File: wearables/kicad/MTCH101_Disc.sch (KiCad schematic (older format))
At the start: 15 parts, among them U1 MTCH101_PKG

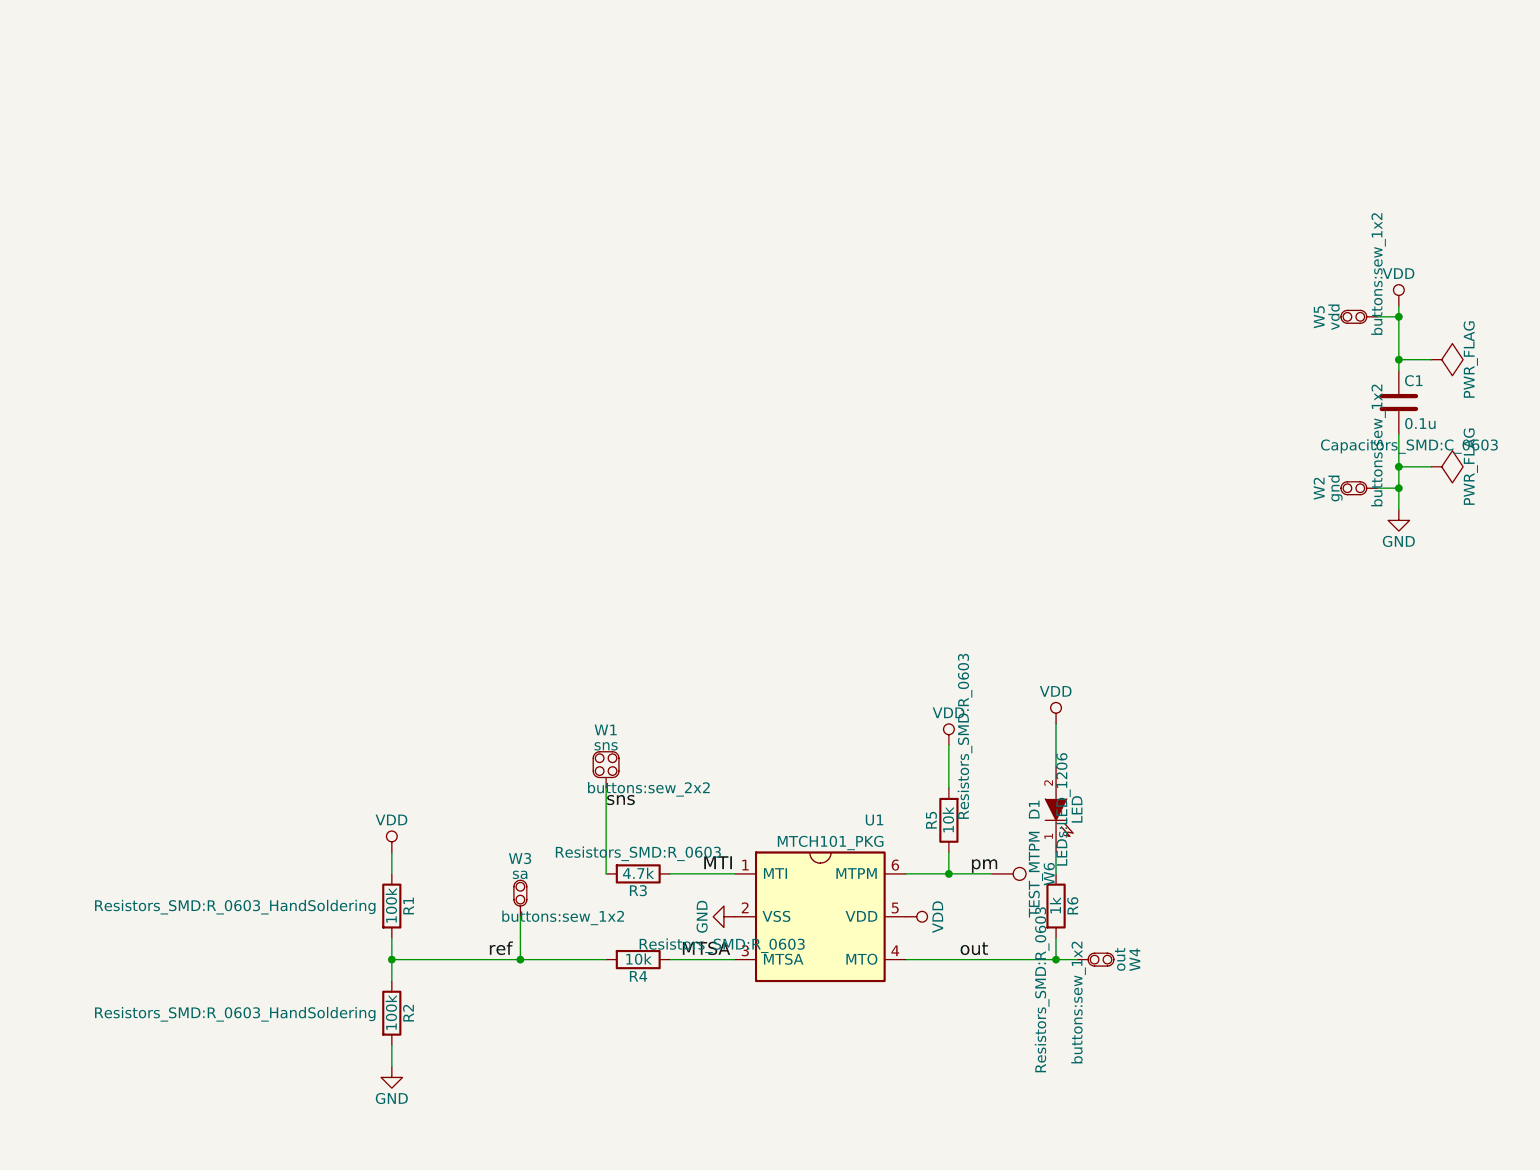
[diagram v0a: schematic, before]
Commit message: more dabbling
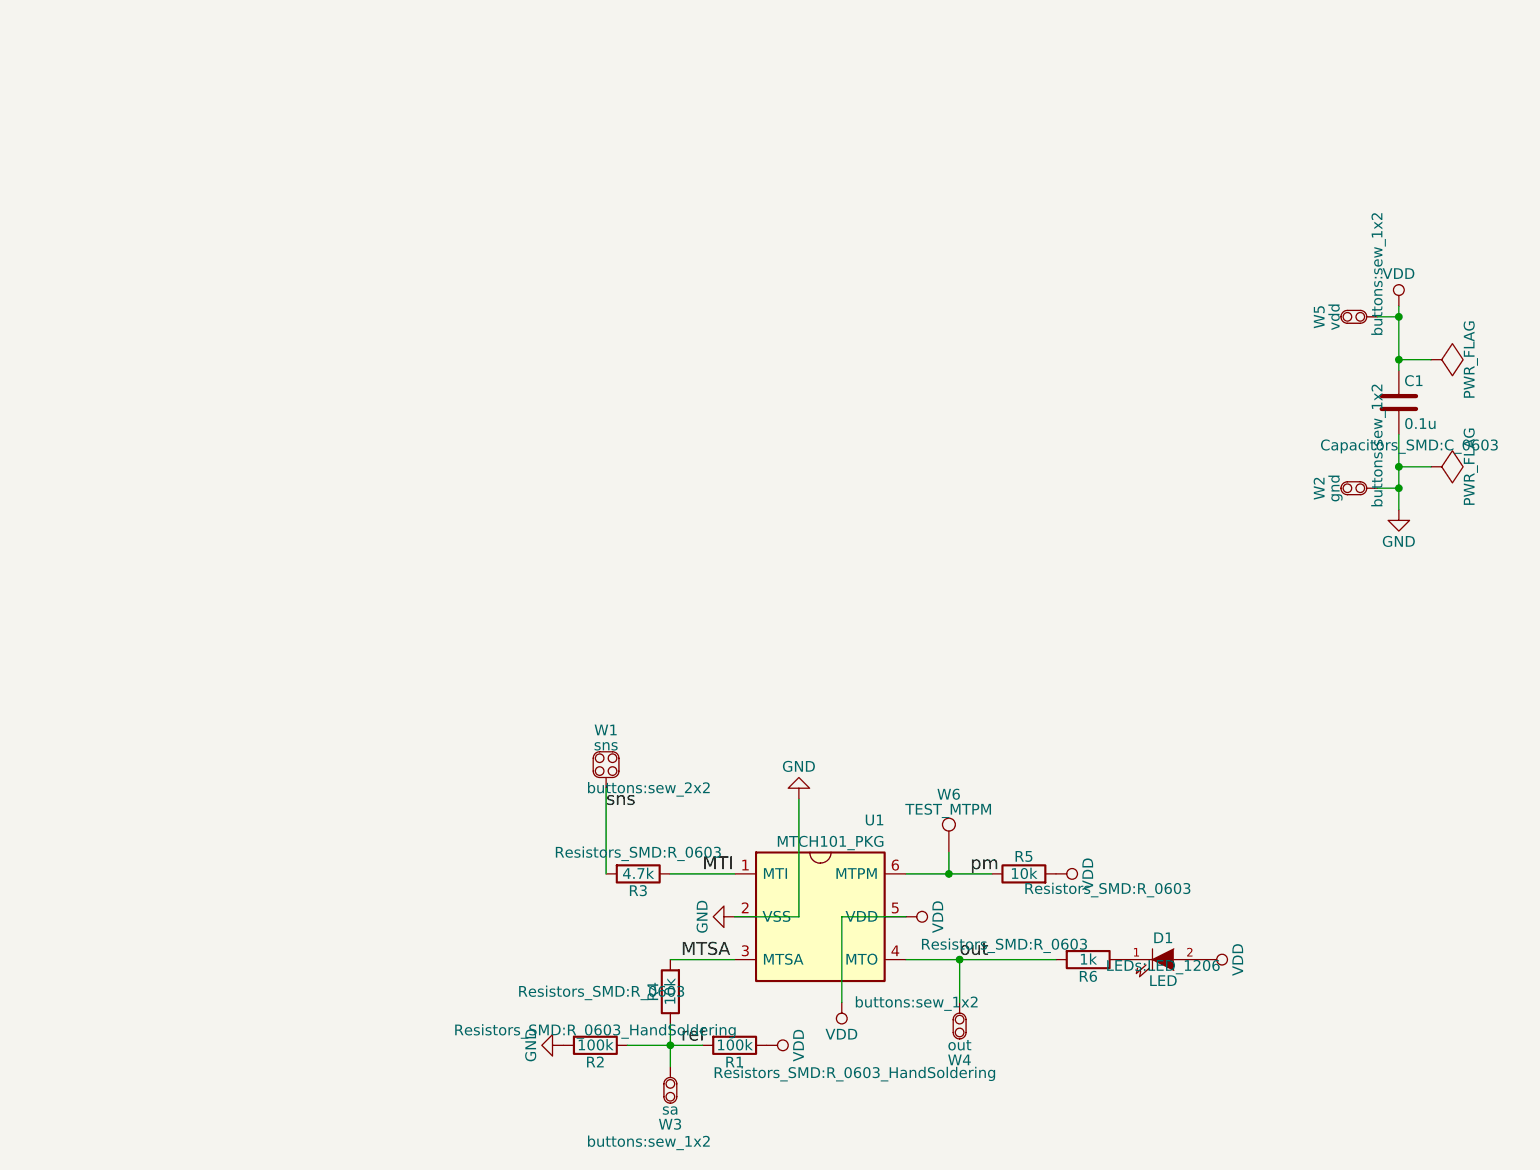
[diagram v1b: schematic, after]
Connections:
- net MTSA: now also R4.2; no longer R4.1
- net ref: now also R4.1; no longer R4.2
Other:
- moved on the sheet: D1, R1, R2, R4, R5, R6, W3, W4, W6
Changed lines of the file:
@@
 L R R4
 U 1 1 58064DD0
-P 3450 5600
-F 0 "R4" V 3530 5600 50  0000 C CNN
-F 1 "10k" V 3450 5600 50  0000 C CNN
-F 2 "Resistors_SMD:R_0603" V 3380 5600 50  0000 L CNN
-F 3 "" H 3450 5600 50  0000 C CNN
-	1    3450 5600
-	0    1    1    0
+P 3600 5750
+F 0 "R4" V 3680 5750 50  0000 C CNN
+F 1 "10k" V 3600 5750 50  0000 C CNN
+F 2 "Resistors_SMD:R_0603" H 3530 5750 50  0000 L CNN
+F 3 "" H 3600 5750 50  0000 C CNN
+	1    3600 5750
+	-1   0    0    1
 $EndComp
 $Comp
 L R R5
 U 1 1 58064FBC
-P 4900 4950
-F 0 "R5" V 4980 4950 50  0000 C CNN
-F 1 "10k" V 4900 4950 50  0000 C CNN
-F 2 "Resistors_SMD:R_0603" V 4830 4950 50  0000 R CNN
-F 3 "" H 4900 4950 50  0000 C CNN
-	1    4900 4950
-	-1   0    0    1
+P 5250 5200
+F 0 "R5" V 5330 5200 50  0000 C CNN
+F 1 "10k" V 5250 5200 50  0000 C CNN
+F 2 "Resistors_SMD:R_0603" V 5180 5200 50  0000 R CNN
+F 3 "" H 5250 5200 50  0000 C CNN
+	1    5250 5200
+	0    -1   -1   0
 $EndComp
 $Comp
 L R R1
 U 1 1 580650CE
-P 2300 5350
-F 0 "R1" V 2380 5350 50  0000 C CNN
-F 1 "100k" V 2300 5350 50  0000 C CNN
-F 2 "Resistors_SMD:R_0603_HandSoldering" H 2230 5350 50  0000 R CNN
-F 3 "" H 2300 5350 50  0000 C CNN
-	1    2300 5350
-	1    0    0    -1
+P 3900 6000
+F 0 "R1" V 3980 6000 50  0000 C CNN
+F 1 "100k" V 3900 6000 50  0000 C CNN
+F 2 "Resistors_SMD:R_0603_HandSoldering" V 4000 5900 50  0000 L TNN
+F 3 "" H 3900 6000 50  0000 C CNN
+	1    3900 6000
+	0    1    1    0
 $EndComp
 $Comp
 L R R2
 U 1 1 580650FF
-P 2300 5850
-F 0 "R2" V 2380 5850 50  0000 C CNN
-F 1 "100k" V 2300 5850 50  0000 C CNN
-F 2 "Resistors_SMD:R_0603_HandSoldering" H 2230 5850 50  0000 R CNN
-F 3 "" H 2300 5850 50  0000 C CNN
-	1    2300 5850
-	1    0    0    -1
+P 3250 6000
+F 0 "R2" V 3330 6000 50  0000 C CNN
+F 1 "100k" V 3250 6000 50  0000 C CNN
+F 2 "Resistors_SMD:R_0603_HandSoldering" V 3180 6000 50  0000 C CNN
+F 3 "" H 3250 6000 50  0000 C CNN
+	1    3250 6000
+	0    1    1    0
 $EndComp
 $Comp
@@
 L R R6
 U 1 1 58065673
-P 5400 5350
-F 0 "R6" V 5480 5350 50  0000 C CNN
-F 1 "1k" V 5400 5350 50  0000 C CNN
-F 2 "Resistors_SMD:R_0603" V 5330 5350 50  0000 R CNN
-F 3 "" H 5400 5350 50  0000 C CNN
-	1    5400 5350
-	1    0    0    -1
+P 5550 5600
+F 0 "R6" V 5630 5600 50  0000 C CNN
+F 1 "1k" V 5550 5600 50  0000 C CNN
+F 2 "Resistors_SMD:R_0603" V 5480 5600 50  0000 R CNN
+F 3 "" H 5550 5600 50  0000 C CNN
+	1    5550 5600
+	0    1    1    0
 $EndComp
 $Comp
 L LED D1
 U 1 1 5806579A
-P 5400 4900
-F 0 "D1" H 5400 5000 50  0000 C CNN
-F 1 "LED" H 5400 4800 50  0000 C CNN
-F 2 "LEDs:LED_1206" H 5400 4900 50  0000 C TNN
-F 3 "" H 5400 4900 50  0000 C CNN
-	1    5400 4900
-	0    -1   -1   0
+P 5900 5600
+F 0 "D1" H 5900 5700 50  0000 C CNN
+F 1 "LED" H 5900 5500 50  0000 C CNN
+F 2 "LEDs:LED_1206" H 5900 5600 50  0000 C TNN
+F 3 "" H 5900 5600 50  0000 C CNN
+	1    5900 5600
+	1    0    0    -1
 $EndComp
 Text Label 4950 5600 0    60   ~ 0
@@
 Text Label 3300 4900 0    60   ~ 0
 sns
-Text Label 2750 5600 0    60   ~ 0
+Text Label 3650 6000 0    60   ~ 0
 ref
 $Comp
 L TEST_1P W6
 U 1 1 580662C8
-P 5100 5200
-F 0 "W6" H 5100 5470 50  0000 C CNN
-F 1 "TEST_MTPM" H 5100 5400 50  0000 C CNN
-F 2 "Measurement_Points:Measurement_Point_Round-SMD-Pad_Small" H 5300 5200 50  0001 C CNN
-F 3 "" H 5300 5200 50  0000 C CNN
-	1    5100 5200
-	0    1    1    0
+P 4900 5100
+F 0 "W6" H 4900 5370 50  0000 C CNN
+F 1 "TEST_MTPM" H 4900 5300 50  0000 C CNN
+F 2 "Measurement_Points:Measurement_Point_Round-SMD-Pad_Small" H 5100 5100 50  0001 C CNN
+F 3 "" H 5100 5100 50  0000 C CNN
+	1    4900 5100
+	1    0    0    -1
 $EndComp
 $Comp
 L VDD #vdd03
 U 1 1 58067C71
-P 5400 4500
-F 0 "#vdd03" H 5400 4350 50  0001 C CNN
-F 1 "VDD" H 5400 4650 50  0000 C CNN
-F 2 "" H 5400 4500 50  0000 C CNN
-F 3 "" H 5400 4500 50  0000 C CNN
-	1    5400 4500
-	1    0    0    -1
+P 6100 5600
+F 0 "#vdd03" H 6100 5450 50  0001 C CNN
+F 1 "VDD" H 6100 5750 50  0000 C CNN
+F 2 "" H 6100 5600 50  0000 C CNN
+F 3 "" H 6100 5600 50  0000 C CNN
+	1    6100 5600
+	0    1    1    0
 $EndComp
 $Comp
 L VDD #vdd04
 U 1 1 580681E5
-P 4900 4600
-F 0 "#vdd04" H 4900 4450 50  0001 C CNN
-F 1 "VDD" H 4900 4750 50  0000 C CNN
-F 2 "" H 4900 4600 50  0000 C CNN
-F 3 "" H 4900 4600 50  0000 C CNN
-	1    4900 4600
-	1    0    0    -1
+P 5400 5200
+F 0 "#vdd04" H 5400 5050 50  0001 C CNN
+F 1 "VDD" H 5400 5350 50  0000 C CNN
+F 2 "" H 5400 5200 50  0000 C CNN
+F 3 "" H 5400 5200 50  0000 C CNN
+	1    5400 5200
+	0    1    1    0
 $EndComp
 $Comp
@@
 L VDD #vdd06
 U 1 1 58068249
-P 2300 5100
-F 0 "#vdd06" H 2300 4950 50  0001 C CNN
-F 1 "VDD" H 2300 5250 50  0000 C CNN
-F 2 "" H 2300 5100 50  0000 C CNN
-F 3 "" H 2300 5100 50  0000 C CNN
-	1    2300 5100
-	1    0    0    -1
+P 4050 6000
+F 0 "#vdd06" H 4050 5850 50  0001 C CNN
+F 1 "VDD" H 4050 6150 50  0000 C CNN
+F 2 "" H 4050 6000 50  0000 C CNN
+F 3 "" H 4050 6000 50  0000 C CNN
+	1    4050 6000
+	0    1    1    0
 $EndComp
 $Comp
@@
 L GND #gnd08
 U 1 1 580686F1
-P 2300 6100
-F 0 "#gnd08" H 2300 5850 50  0001 C CNN
-F 1 "GND" H 2300 5950 50  0000 C CNN
-F 2 "" H 2300 6100 50  0000 C CNN
-F 3 "" H 2300 6100 50  0000 C CNN
-	1    2300 6100
-	1    0    0    -1
+P 3100 6000
+F 0 "#gnd08" H 3100 5750 50  0001 C CNN
+F 1 "GND" H 3100 5850 50  0000 C CNN
+F 2 "" H 3100 6000 50  0000 C CNN
+F 3 "" H 3100 6000 50  0000 C CNN
+	1    3100 6000
+	0    1    1    0
 $EndComp
 $Comp
@@
 	4700 5200 5100 5200
 Wire Wire Line
-	2300 5500 2300 5700
-Wire Wire Line
-	2300 5600 3300 5600
-Connection ~ 2300 5600
-Wire Wire Line
-	2300 5100 2300 5200
-Wire Wire Line
-	2300 6000 2300 6100
-Wire Wire Line
-	5400 5600 5400 5500
-Wire Wire Line
-	5400 5100 5400 5200
-Wire Wire Line
-	5400 4500 5400 4700
-Wire Wire Line
-	4700 5600 5500 5600
-Connection ~ 5400 5600
-Wire Wire Line
-	4900 4600 4900 4800
+	4700 5600 5400 5600
 Wire Wire Line
 	4900 5100 4900 5200
 Connection ~ 4900 5200
-Wire Wire Line
-	2900 5600 2900 5600
-Connection ~ 2900 5600
 Wire Wire Line
 	7150 2800 7000 2800
@@
 Wire Wire Line
 	3600 5600 3900 5600
-Wire Wire Line
-	2900 5400 2900 5600
 $Comp
 L SEW_1X2 W3
 U 1 1 580A30E6
-P 2900 5400
-F 0 "W3" H 2900 5670 50  0000 C CNN
-F 1 "sa" H 2900 5600 50  0000 C CNN
-F 2 "buttons:sew_1x2" H 3100 5400 50  0000 C CNN
-F 3 "" H 3100 5400 50  0000 C CNN
-	1    2900 5400
-	1    0    0    -1
+P 3600 6100
+F 0 "W3" H 3600 6370 50  0000 C CNN
+F 1 "sa" H 3600 6300 50  0000 C CNN
+F 2 "buttons:sew_1x2" H 3700 6450 50  0000 C CNN
+F 3 "" H 3800 6100 50  0000 C CNN
+	1    3600 6100
+	-1   0    0    1
 $EndComp
 $Comp
 L SEW_1X2 W4
 U 1 1 580A3684
-P 5500 5600
-F 0 "W4" H 5500 5870 50  0000 C CNN
-F 1 "out" H 5500 5800 50  0000 C CNN
-F 2 "buttons:sew_1x2" H 5700 5600 50  0000 C CNN
-F 3 "" H 5700 5600 50  0000 C CNN
-	1    5500 5600
-	0    1    1    0
+P 4950 5800
+F 0 "W4" H 4950 6070 50  0000 C CNN
+F 1 "out" H 4950 6000 50  0000 C CNN
+F 2 "buttons:sew_1x2" H 5150 5800 50  0000 C CNN
+F 3 "" H 5150 5800 50  0000 C CNN
+	1    4950 5800
+	-1   0    0    1
 $EndComp
 $Comp
@@
 	0    -1   -1   0
 $EndComp
+Wire Wire Line
+	4950 5800 4950 5600
+Connection ~ 4950 5600
+Wire Wire Line
+	3600 5900 3600 6100
+Wire Wire Line
+	3400 6000 3750 6000
+Connection ~ 3600 6000
+$Comp
+L GND #gnd011
+U 1 1 580A55A8
+P 4200 4850
+F 0 "#gnd011" H 4200 4600 50  0001 C CNN
+F 1 "GND" H 4200 4700 50  0000 C CNN
+F 2 "" H 4200 4850 50  0000 C CNN
+F 3 "" H 4200 4850 50  0000 C CNN
+	1    4200 4850
+	-1   0    0    1
+$EndComp
+Wire Wire Line
+	3900 5400 4200 5400
+Wire Wire Line
+	4200 5400 4200 4850
+$Comp
+L VDD #vdd012
+U 1 1 580A5607
+P 4400 5800
+F 0 "#vdd012" H 4400 5650 50  0001 C CNN
+F 1 "VDD" H 4400 5950 50  0000 C CNN
+F 2 "" H 4400 5800 50  0000 C CNN
+F 3 "" H 4400 5800 50  0000 C CNN
+	1    4400 5800
+	-1   0    0    1
+$EndComp
+Wire Wire Line
+	4700 5400 4400 5400
+Wire Wire Line
+	4400 5400 4400 5800
 $EndSCHEMATC

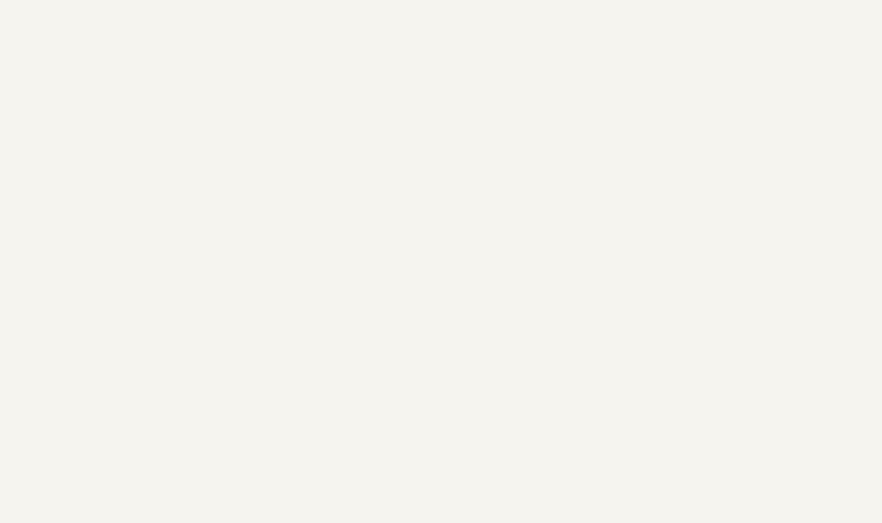
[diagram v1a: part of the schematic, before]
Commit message: More misc play.
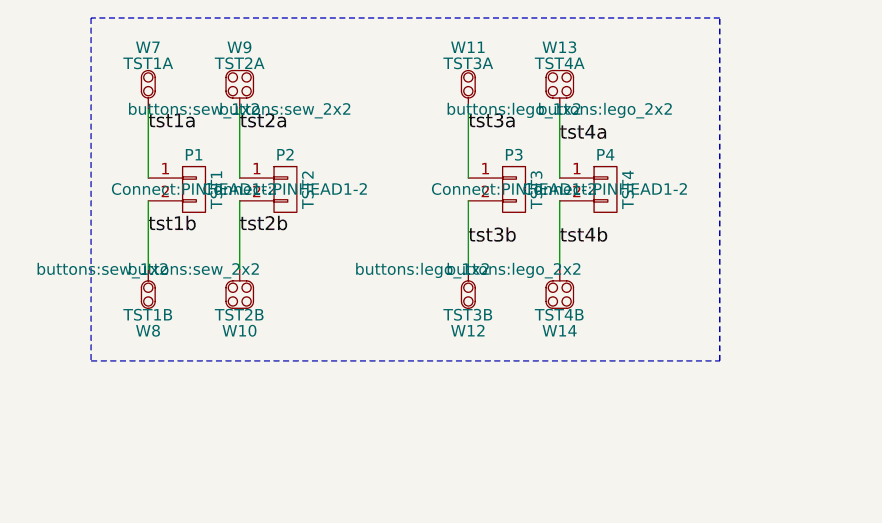
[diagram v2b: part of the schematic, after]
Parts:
- added P1: TST1, Connect:PINHEAD1-2, symbol CONN_01X02
- added P2: TST2, Connect:PINHEAD1-2, symbol CONN_01X02
- added P3: TST3, Connect:PINHEAD1-2, symbol CONN_01X02
- added P4: TST4, Connect:PINHEAD1-2, symbol CONN_01X02
- added W10: TST2B, buttons:sew_2x2, symbol SEW_2X2
- added W11: TST3A, buttons:lego_1x2, symbol SEW_1X2
- added W12: TST3B, buttons:lego_1x2, symbol SEW_1X2
- added W13: TST4A, buttons:lego_2x2, symbol SEW_2X2
- added W14: TST4B, buttons:lego_2x2, symbol SEW_2X2
- added W7: TST1A, buttons:sew_1x2, symbol SEW_1X2
- added W8: TST1B, buttons:sew_1x2, symbol SEW_1X2
- added W9: TST2A, buttons:sew_2x2, symbol SEW_2X2
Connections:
- new net tst1a: P1.1 (P1), W7.1
- new net tst1b: P1.2 (P2), W8.1
- new net tst2a: P2.1 (P1), W9.1
- new net tst2b: P2.2 (P2), W10.1
- new net tst3a: P3.1 (P1), W11.1
- new net tst3b: P3.2 (P2), W12.1
- new net tst4a: P4.1 (P1), W13.1
- new net tst4b: P4.2 (P2), W14.1
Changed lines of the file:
@@
 Wire Wire Line
 	4400 5400 4400 5800
+Wire Notes Line
+	4100 1200 1350 1200
+Wire Notes Line
+	1350 1200 1350 2700
+Wire Notes Line
+	1350 2700 4100 2700
+Wire Notes Line
+	4100 2700 4100 1200
+$Comp
+L SEW_1X2 W7
+U 1 1 580CE257
+P 1600 1600
+F 0 "W7" H 1600 1870 50  0000 C CNN
+F 1 "TST1A" H 1600 1800 50  0000 C CNN
+F 2 "buttons:sew_1x2" H 1800 1600 50  0000 C CNN
+F 3 "" H 1800 1600 50  0000 C CNN
+	1    1600 1600
+	1    0    0    -1
+$EndComp
+$Comp
+L SEW_1X2 W8
+U 1 1 580CE2C7
+P 1600 2300
+F 0 "W8" H 1600 2570 50  0000 C CNN
+F 1 "TST1B" H 1600 2500 50  0000 C CNN
+F 2 "buttons:sew_1x2" H 1800 2300 50  0000 C CNN
+F 3 "" H 1800 2300 50  0000 C CNN
+	1    1600 2300
+	-1   0    0    1
+$EndComp
+$Comp
+L SEW_2X2 W9
+U 1 1 580CE33E
+P 2000 1600
+F 0 "W9" H 2000 1870 50  0000 C CNN
+F 1 "TST2A" H 2000 1800 50  0000 C CNN
+F 2 "buttons:sew_2x2" H 2200 1600 50  0000 C CNN
+F 3 "" H 2200 1600 50  0000 C CNN
+	1    2000 1600
+	1    0    0    -1
+$EndComp
+$Comp
+L SEW_2X2 W10
+U 1 1 580CE39E
+P 2000 2300
+F 0 "W10" H 2000 2570 50  0000 C CNN
+F 1 "TST2B" H 2000 2500 50  0000 C CNN
+F 2 "buttons:sew_2x2" H 2200 2300 50  0000 C CNN
+F 3 "" H 2200 2300 50  0000 C CNN
+	1    2000 2300
+	-1   0    0    1
+$EndComp
+Wire Wire Line
+	1600 1600 1600 1900
+Wire Wire Line
+	2000 1600 2000 1900
+Wire Wire Line
+	2000 2000 2000 2300
+Wire Wire Line
+	1600 2000 1600 2300
+$Comp
+L CONN_01X02 P1
+U 1 1 580CE890
+P 1800 1950
+F 0 "P1" H 1800 2100 50  0000 C CNN
+F 1 "TST1" V 1900 1950 50  0000 C CNN
+F 2 "Connect:PINHEAD1-2" H 1800 1950 50  0000 C CNN
+F 3 "" H 1800 1950 50  0000 C CNN
+	1    1800 1950
+	1    0    0    -1
+$EndComp
+$Comp
+L CONN_01X02 P2
+U 1 1 580CE8EA
+P 2200 1950
+F 0 "P2" H 2200 2100 50  0000 C CNN
+F 1 "TST2" V 2300 1950 50  0000 C CNN
+F 2 "Connect:PINHEAD1-2" H 2200 1950 50  0000 C CNN
+F 3 "" H 2200 1950 50  0000 C CNN
+	1    2200 1950
+	1    0    0    -1
+$EndComp
+$Comp
+L SEW_1X2 W11
+U 1 1 580CF0AD
+P 3000 1600
+F 0 "W11" H 3000 1870 50  0000 C CNN
+F 1 "TST3A" H 3000 1800 50  0000 C CNN
+F 2 "buttons:lego_1x2" H 3200 1600 50  0000 C CNN
+F 3 "" H 3200 1600 50  0000 C CNN
+	1    3000 1600
+	1    0    0    -1
+$EndComp
+$Comp
+L SEW_1X2 W12
+U 1 1 580CF0B3
+P 3000 2300
+F 0 "W12" H 3000 2570 50  0000 C CNN
+F 1 "TST3B" H 3000 2500 50  0000 C CNN
+F 2 "buttons:lego_1x2" H 3200 2300 50  0000 C CNN
+F 3 "" H 3200 2300 50  0000 C CNN
+	1    3000 2300
+	-1   0    0    1
+$EndComp
+$Comp
+L SEW_2X2 W13
+U 1 1 580CF0B9
+P 3400 1600
+F 0 "W13" H 3400 1870 50  0000 C CNN
+F 1 "TST4A" H 3400 1800 50  0000 C CNN
+F 2 "buttons:lego_2x2" H 3600 1600 50  0000 C CNN
+F 3 "" H 3600 1600 50  0000 C CNN
+	1    3400 1600
+	1    0    0    -1
+$EndComp
+$Comp
+L SEW_2X2 W14
+U 1 1 580CF0BF
+P 3400 2300
+F 0 "W14" H 3400 2570 50  0000 C CNN
+F 1 "TST4B" H 3400 2500 50  0000 C CNN
+F 2 "buttons:lego_2x2" H 3600 2300 50  0000 C CNN
+F 3 "" H 3600 2300 50  0000 C CNN
+	1    3400 2300
+	-1   0    0    1
+$EndComp
+Wire Wire Line
+	3000 1600 3000 1900
+Wire Wire Line
+	3400 1600 3400 1900
+Wire Wire Line
+	3400 2000 3400 2300
+Wire Wire Line
+	3000 2000 3000 2300
+$Comp
+L CONN_01X02 P3
+U 1 1 580CF0C9
+P 3200 1950
+F 0 "P3" H 3200 2100 50  0000 C CNN
+F 1 "TST3" V 3300 1950 50  0000 C CNN
+F 2 "Connect:PINHEAD1-2" H 3200 1950 50  0000 C CNN
+F 3 "" H 3200 1950 50  0000 C CNN
+	1    3200 1950
+	1    0    0    -1
+$EndComp
+$Comp
+L CONN_01X02 P4
+U 1 1 580CF0CF
+P 3600 1950
+F 0 "P4" H 3600 2100 50  0000 C CNN
+F 1 "TST4" V 3700 1950 50  0000 C CNN
+F 2 "Connect:PINHEAD1-2" H 3600 1950 50  0000 C CNN
+F 3 "" H 3600 1950 50  0000 C CNN
+	1    3600 1950
+	1    0    0    -1
+$EndComp
+Text Label 1600 1700 0    60   ~ 0
+tst1a
+Text Label 1600 2150 0    60   ~ 0
+tst1b
+Text Label 2000 1700 0    60   ~ 0
+tst2a
+Text Label 2000 2150 0    60   ~ 0
+tst2b
+Text Label 3000 1700 0    60   ~ 0
+tst3a
+Text Label 3000 2200 0    60   ~ 0
+tst3b
+Text Label 3400 1750 0    60   ~ 0
+tst4a
+Text Label 3400 2200 0    60   ~ 0
+tst4b
 $EndSCHEMATC
